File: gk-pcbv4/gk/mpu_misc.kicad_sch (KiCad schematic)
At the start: 30 parts, among them J10 Conn_ARM_JTAG_SWD_10, J14 Conn_01x03, J5 Conn_ARM_Cortex_Debug_ETM_20, SW1 SW_Push, SW2 DS04-254-[12]-04BK-SMT, U5 STM32MP255DAI3, Y1 24MHz, Y2 CM8V-T1A-32.768kHz-12.5pF-20P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

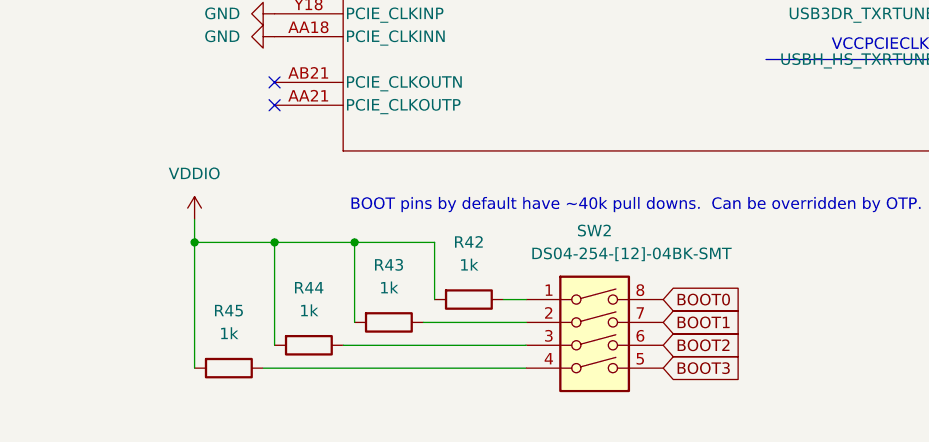
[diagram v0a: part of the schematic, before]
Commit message: pcb order 20251115
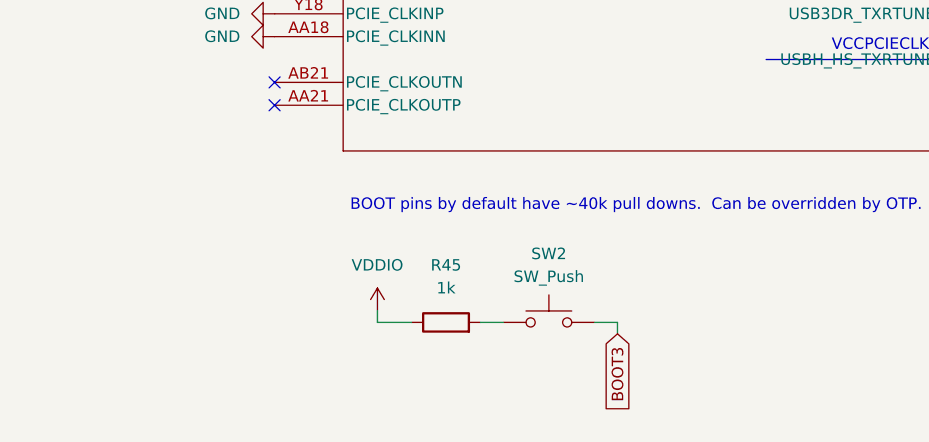
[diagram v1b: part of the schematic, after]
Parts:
- removed R42, R43, R44: 1k, Resistor_SMD:R_0603_1608Metric, symbol Device:R
- removed SW2: DS04-254-[12]-04BK-SMT, Button_Switch_SMD:SW_DIP_SPSTx04_Slide_9.78x12.34mm_W8.61mm_P2.54mm, symbol Switch:SW_DIP_x04
- added SW2: SW_Push, Button_Switch_SMD:SW_SPST_PTS647_Sx38, symbol Switch:SW_Push
- SW1: footprint gk-pcbv3:Tactile Switch 6x3.5mm -> Button_Switch_SMD:SW_SPST_PTS647_Sx38
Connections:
- net BOOT3: now also SW2.2
- net VDDIO: now also R45.1; no longer R45.2
- new net: R45.2, SW2.1
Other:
- moved on the sheet: R45
